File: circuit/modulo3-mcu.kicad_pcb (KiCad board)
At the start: 2 copper layers, 87 x 52 mm, 35 parts, among them Q1 BS250, U1 74LVC2G32DC, U10 PWR_CONN, U2 AVR64DA64, U3 SN74LVC1G17, U4 UPDI, U5 TOUCHSCREEN_240x320, U6 FV1_CONN, U7 DBG_UART, U8 AMPCTRL, Y1 32768Hz

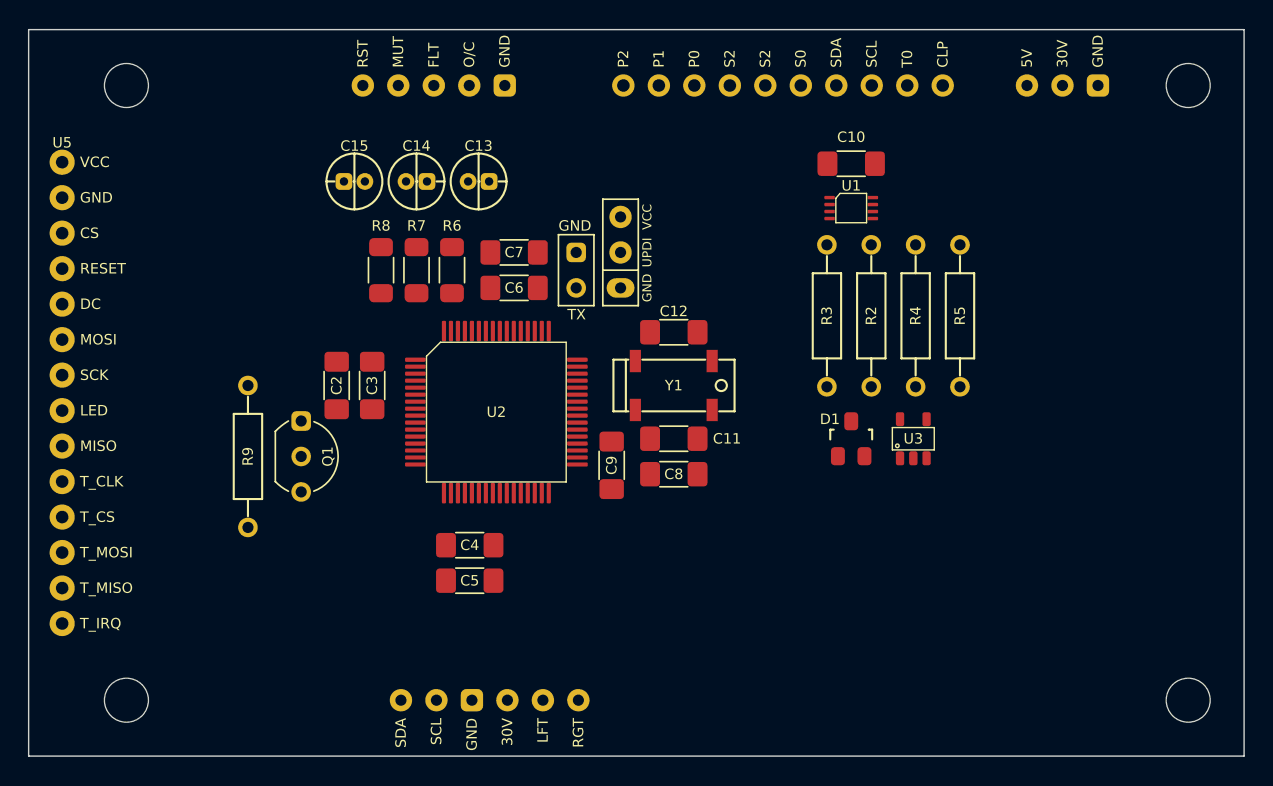
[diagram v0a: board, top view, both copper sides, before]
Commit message: lotsa things :)
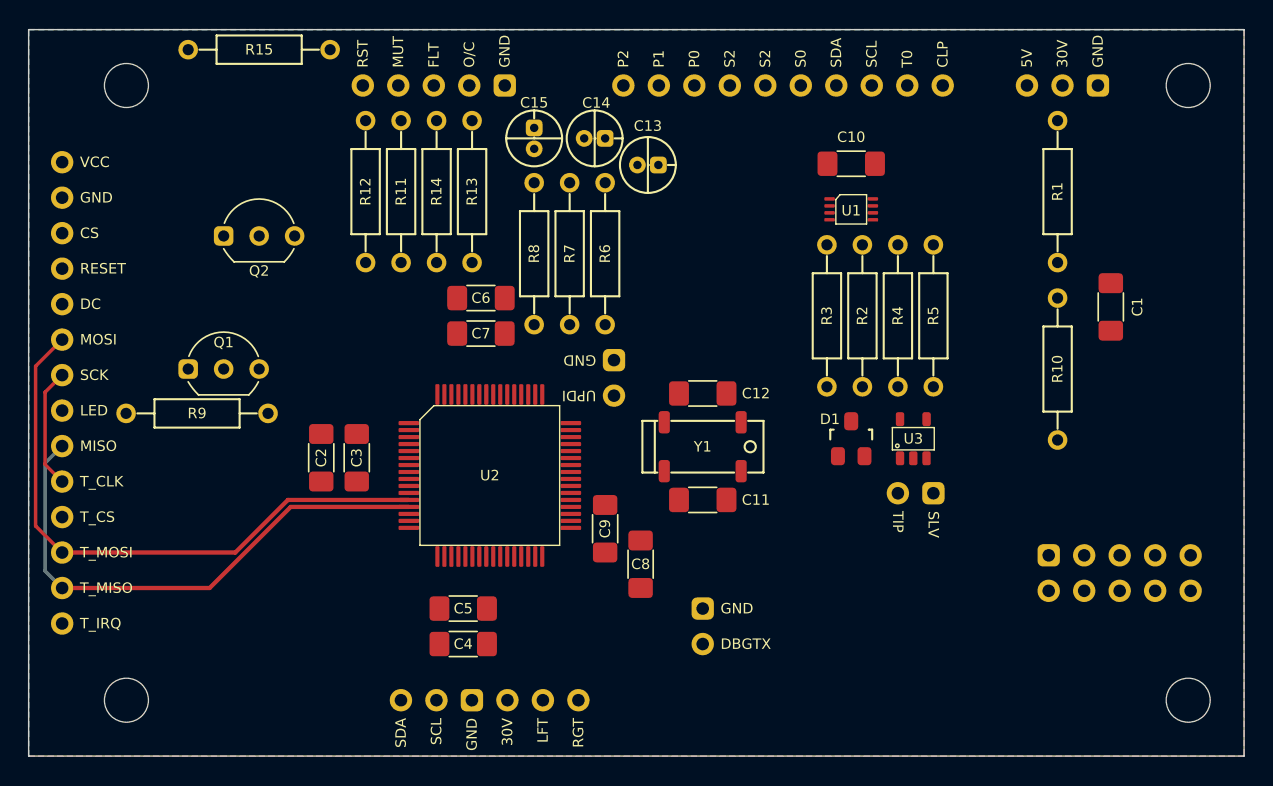
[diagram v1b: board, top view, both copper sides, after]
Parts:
- added C1: 10n, myAmp:C_1206, F.Cu at (124.5, 69.8)
- added Q2: BS170, myAmp:TO-92_Inline_Wide, F.Cu at (63.5, 64.8)
- added R1: 10k, myAmp:R_10MM, F.Cu at (120.7, 61.6)
- added R10: 1k, myAmp:R_10MM, F.Cu at (120.7, 74.3)
- added R11: 10k, myAmp:R_10MM, F.Cu at (73.7, 61.6)
- added R12: 100, myAmp:R_10MM, F.Cu at (71.1, 61.6)
- added R13: 100, myAmp:R_10MM, F.Cu at (78.7, 61.6)
- added R14: 100, myAmp:R_10MM, F.Cu at (76.2, 61.6)
- added R15: 10k, myAmp:R_10MM, F.Cu at (63.5, 51.4)
- added U11: FOOTSWITCH, myAmp:FOOTSWITCH, F.Cu at (111.8, 83.2)
- added U12: ~, myAmp:KNOBS, F.Cu at (125.1, 88.9)
- R6, R7, R8: footprint myAmp:R_1206 -> myAmp:R_10MM
- moved U7 27.1 mm to (95.2, 92.7)
- moved C15 13.2 mm to (83.2, 57.8), turned to 90 degrees
- moved C14 13.1 mm to (87.5, 57.8)
- moved C13 12.2 mm to (91.3, 59.7)
- moved R6 11.0 mm to (88.3, 66.0)
- moved R7 11.0 mm to (85.7, 66.0)
- moved R8 11.0 mm to (83.2, 66.0)
- moved Q1 8.36 mm to (61.0, 74.3), turned to 0 degrees
- moved U4 7.73 mm to (88.9, 73.7), turned to 180 degrees
- moved C4 7.09 mm to (78.1, 94.0)
- moved C8 6.86 mm to (90.8, 88.3), turned to -90 degrees
- moved C7 6.27 mm to (79.4, 71.8)
- moved C2 5.29 mm to (67.9, 80.6)
- moved C3 5.29 mm to (70.5, 80.6)
- moved C11 4.85 mm to (95.2, 83.7)
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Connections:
- U10 pad 1: unconnected-(U10-GND-Pad1) -> GND
- U10 pad 2: unconnected-(U10-30V-Pad2) -> Net-(U10-30V)
- U10 pad 3: unconnected-(U10-5V-Pad3) -> +5V
- U2 pad 1: /T_IRQ -> unconnected-(U2-PA3-Pad1)
- U2 pad 10: /S_CS -> unconnected-(U2-PB2-Pad10)
- U2 pad 11: /S_LED -> unconnected-(U2-PB3-Pad11)
- U2 pad 12: unconnected-(U2-PB4-Pad12) -> /S_MOSI
- U2 pad 13: unconnected-(U2-PB5-Pad13) -> /S_MISO
- U2 pad 14: unconnected-(U2-PB6-Pad14) -> /S_SCK
- U2 pad 15: unconnected-(U2-PB7-Pad15) -> /T_IRQ
- U2 pad 18: unconnected-(U2-PC2-Pad18) -> /MIX_SDA
- U2 pad 19: unconnected-(U2-PC3-Pad19) -> /MIX_SCL
- U2 pad 2: /S_MOSI -> unconnected-(U2-PA4-Pad2)
- U2 pad 3: /S_MISO -> unconnected-(U2-PA5-Pad3)
- U2 pad 4: /S_SCK -> unconnected-(U2-PA6-Pad4)
- U2 pad 46: unconnected-(U2-PF2-Pad46) -> /FV_SDA
- U2 pad 47: unconnected-(U2-PF3-Pad47) -> /FV_SCL
- U2 pad 48: unconnected-(U2-PF4-Pad48) -> /S0
- U2 pad 49: unconnected-(U2-PF5-Pad49) -> /S1
- U2 pad 5: /T_CS -> unconnected-(U2-PA7-Pad5)
- U2 pad 50: unconnected-(U2-(~{RESET})PF6-Pad50) -> /S2
- U2 pad 52: /DBG_TX -> /PWM0
- U2 pad 53: unconnected-(U2-PG1-Pad53) -> /PWM1
- U2 pad 54: unconnected-(U2-PG2-Pad54) -> /PWM2
- U2 pad 58: unconnected-(U2-PG4-Pad58) -> /OTW_CLIP
- U2 pad 59: unconnected-(U2-PG5-Pad59) -> /FAULT
- U2 pad 60: unconnected-(U2-PG6-Pad60) -> /POW_RESET
- U2 pad 62: /PWM0 -> unconnected-(U2-PA0(EXTCLK)-Pad62)
- U2 pad 63: /PWM1 -> unconnected-(U2-PA1-Pad63)
- U2 pad 64: /PWM2 -> unconnected-(U2-PA2-Pad64)
- U2 pad 8: /S_DC -> unconnected-(U2-PB0-Pad8)
- U2 pad 9: /S_RST -> unconnected-(U2-PB1-Pad9)
- U5 pad 1: /T_IRQ -> +3.3V
- U5 pad 10: /S_DC -> /S_SCK
- U5 pad 11: /S_RST -> /T_CS
- U5 pad 12: /S_CS -> /S_MOSI
- U5 pad 13: GND -> /S_MISO
- U5 pad 14: +3.3V -> /T_IRQ
- U5 pad 2: /S_MISO -> GND
- U5 pad 3: /S_MOSI -> /S_CS
- U5 pad 4: /T_CS -> /S_RST
- U5 pad 5: /S_SCK -> /S_DC
- U5 pad 6: /S_MISO -> /S_MOSI
- U5 pad 7: Net-(U5-LED) -> /S_SCK
- U5 pad 8: /S_SCK -> Net-(U5-LED)
- U5 pad 9: /S_MOSI -> /S_MISO
- U8 pad 1: unconnected-(U8-GND-Pad1) -> GND
- U8 pad 2: unconnected-(U8-RESET-Pad2) -> Net-(U8-RESET)
- U8 pad 3: unconnected-(U8-MUTE-Pad3) -> /MUTE
- U8 pad 4: unconnected-(U8-FAULT-Pad4) -> Net-(U8-FAULT)
- U8 pad 5: unconnected-(U8-OTW_CLIP-Pad5) -> Net-(U8-OTW_CLIP)
- U9 pad 1: unconnected-(U9-SDA-Pad1) -> /MIX_SDA
- U9 pad 2: unconnected-(U9-SCL-Pad2) -> /MIX_SCL
- U9 pad 3: unconnected-(U9-GND-Pad3) -> GND
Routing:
- net /S_MOSI: track 0.00 -> 43.2 mm
- net /S_MISO: track 0.00 -> 38.4 mm
- net /S_SCK: track 0.00 -> 8.63 mm
- added copper zone on B.Cu, net GND
- added copper zone on F.Cu, net GND
